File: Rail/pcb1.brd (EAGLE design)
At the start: 49.7 x 86.4 mm, 46 parts, among them J6 638207222005, J7 638207222005, U4 TLE9250VSJ, X1 S4P-VH

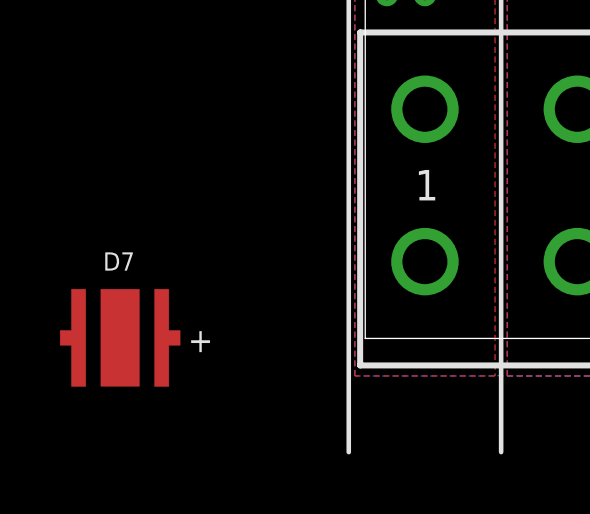
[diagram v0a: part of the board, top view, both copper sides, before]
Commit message: therm
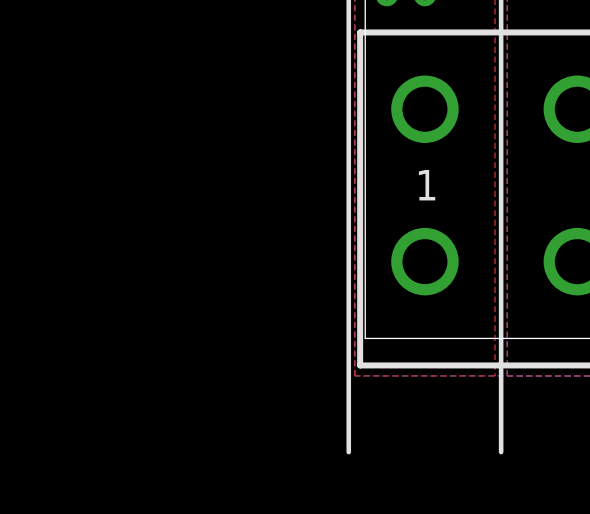
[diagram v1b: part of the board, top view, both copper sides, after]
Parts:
- removed D7: 150353GS74500, LED:WL-SMDC_3535
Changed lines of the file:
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@@
 <attribute name="VALUE" x="-14.9116" y="-0.9442" size="0.8128" layer="27" align="bottom-right"/>
-</element>
-<element name="D7" library="LED" package="WL-SMDC_3535" package3d_urn="urn:adsk.eagle:package:19063445/2" value="150353GS74500" x="-33.02" y="-43.18" smashed="yes">
-<attribute name="CHIP-TECHNOLOGY" value="InGaN" x="-33.02" y="-43.18" size="1.778" layer="27" display="off"/>
-<attribute name="DATASHEET-URL" value="https://www.we-online.com/catalog/datasheet/150353GS74500.pdf" x="-33.02" y="-43.18" size="1.778" layer="27" display="off"/>
-<attribute name="EMITTING-COLOR" value="Green" x="-33.02" y="-43.18" size="1.778" layer="27" display="off"/>
-<attribute name="LAMDA-DOM-TYP" value="525nm" x="-33.02" y="-43.18" size="1.778" layer="27" display="off"/>
-<attribute name="LAMDA-PEAK-TYP" value="520nm" x="-33.02" y="-43.18" size="1.778" layer="27" display="off"/>
-<attribute name="NAME" x="-33.06" y="-40.94" size="0.6096" layer="25" align="bottom-center"/>
-<attribute name="PART-NUMBER" value="150353GS74500" x="-33.02" y="-43.18" size="1.778" layer="27" display="off"/>
-<attribute name="PHI-V-TYP" value="85lm" x="-33.02" y="-43.18" size="1.778" layer="27" display="off"/>
-<attribute name="V-F-TYP" value="3.4V" x="-33.02" y="-43.18" size="1.778" layer="27" display="off"/>
-<attribute name="VALUE" x="-33.29" y="-45.99" size="0.6096" layer="27" align="bottom-center"/>
-<attribute name="VIEWING-ANGLE" value="125°" x="-33.02" y="-43.18" size="1.778" layer="27" display="off"/>
 </element>
 </elements>
